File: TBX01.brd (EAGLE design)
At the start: 49.8 x 40.1 mm, 74 parts, among them IC1 TPS62120, U3 STM32L151CCT6, U6 MCP73833, X2 FH12-10S-0.5SH, Y1 CRYSTAL.ABS07

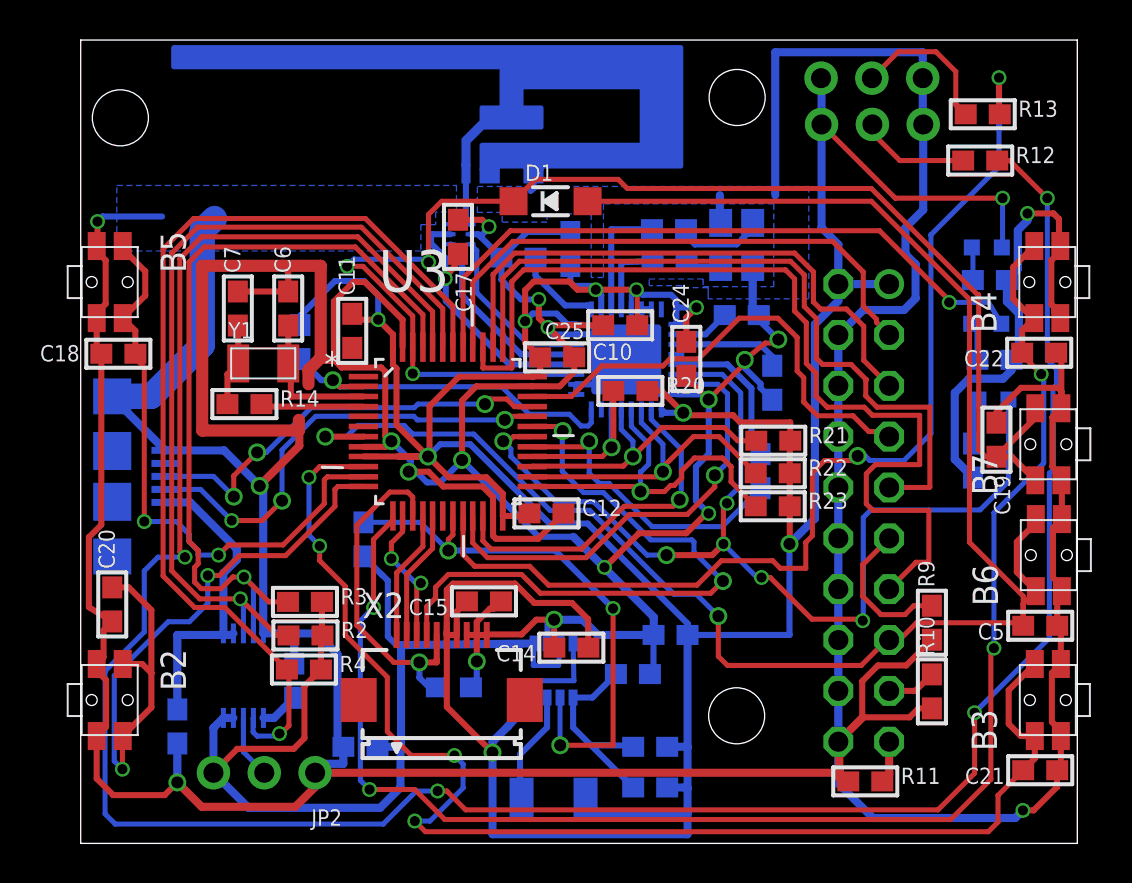
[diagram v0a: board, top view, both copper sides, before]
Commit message: TBX01 v0.4-r201508241723
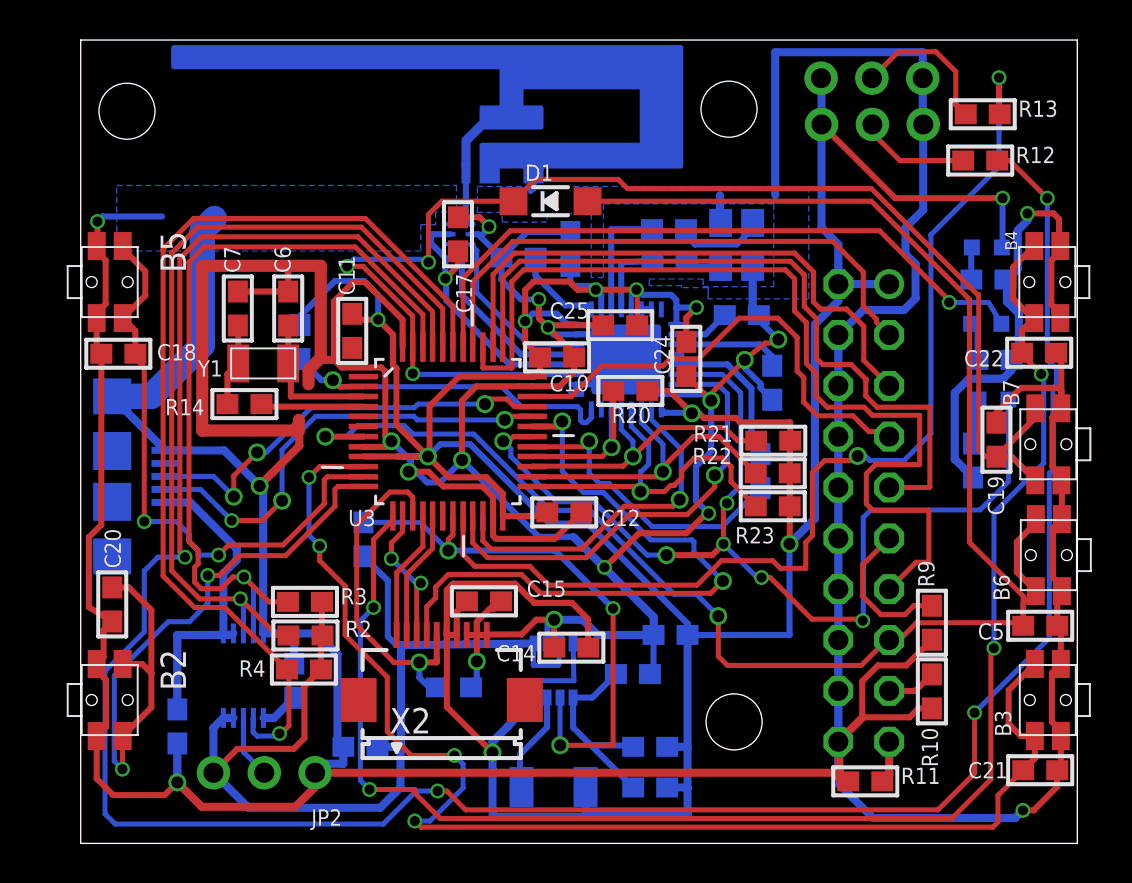
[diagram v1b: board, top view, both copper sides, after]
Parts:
- moved C12 0.89 mm to (24.2, 16.5)
- moved L1 0.53 mm to (23.6, 2.82)
- moved C17 0.13 mm to (18.8, 30.4)
- moved R8 0.08 mm to (45.3, 28.2)
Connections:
- net TP: now also U1.GND; no longer U1.33
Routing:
- net GND: track 427.3 -> 428.8 mm
